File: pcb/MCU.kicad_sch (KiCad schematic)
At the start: 14 parts, among them U1 WeMos_S2_mini

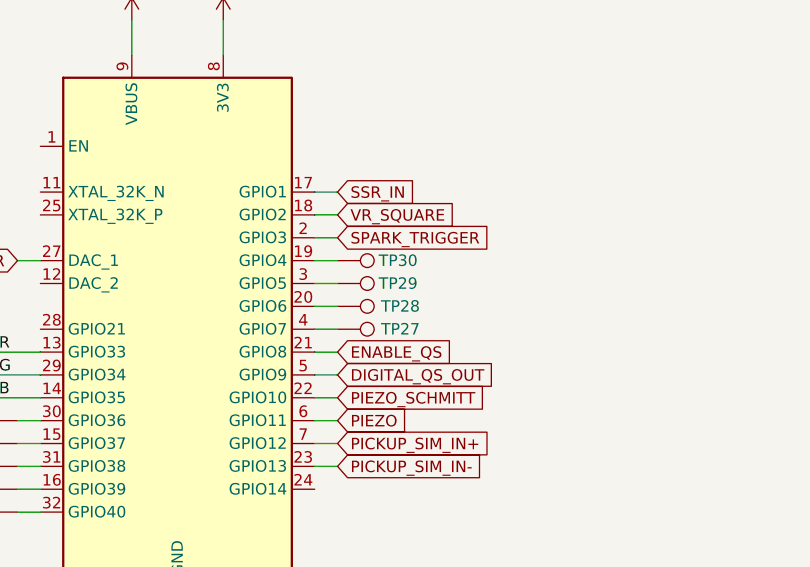
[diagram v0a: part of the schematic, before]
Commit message: added connector and simulation link
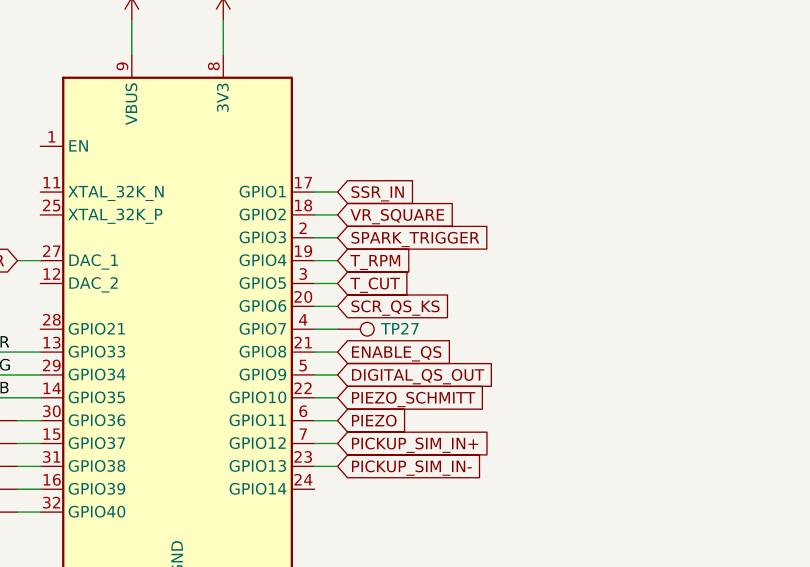
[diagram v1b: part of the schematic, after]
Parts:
- removed TP28, TP29, TP30: TestPoint, Connector_PinHeader_1.00mm:PinHeader_1x01_P1.00mm_Vertical, symbol Connector:TestPoint
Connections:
- net SCR_QS_KS: now reaches U1.20 (GPIO6)
- net T_RPM: now reaches U1.19 (GPIO4)
- net T_CUT: now reaches U1.3 (GPIO5)
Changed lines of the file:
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@@
+		)
+	)
+	(global_label "SCR_QS_KS"
+		(shape input)
+		(at 86.36 64.77 0)
+		(fields_autoplaced yes)
+		(effects
+			(font
+				(size 1.27 1.27)
+			)
+			(justify left)
+		)
+		(property "Intersheetrefs" "${INTERSHEET_REFS}"
+			(at 100.0494 64.77 0)
+			(effects
+				(font
+					(size 1.27 1.27)
+				)
+				(justify left)
+				(hide yes)
+			)
 		)
 	)
@@
 		)
 	)
+	(global_label "T_RPM"
+		(shape input)
+		(at 86.36 59.69 0)
+		(fields_autoplaced yes)
+		(effects
+			(font
+				(size 1.27 1.27)
+			)
+			(justify left)
+		)
+		(property "Intersheetrefs" "${INTERSHEET_REFS}"
+			(at 95.2718 59.69 0)
+			(effects
+				(font
+					(size 1.27 1.27)
+				)
+				(justify left)
+				(hide yes)
+			)
+		)
+	)
+	(global_label "T_CUT"
+		(shape input)
+		(at 86.36 62.23 0)
+		(fields_autoplaced yes)
+		(effects
+			(font
+				(size 1.27 1.27)
+			)
+			(justify left)
+		)
+		(property "Intersheetrefs" "${INTERSHEET_REFS}"
+			(at 94.8485 62.23 0)
+			(effects
+				(font
+					(size 1.27 1.27)
+				)
+				(justify left)
+				(hide yes)
+			)
+		)
+	)
 	(global_label "PWM_VR"
 		(shape input)
@@
 	)
 	(symbol
-		(lib_id "Connector:TestPoint")
-		(at 86.36 64.77 270)
-		(unit 1)
-		(exclude_from_sim no)
-		(in_bom yes)
-		(on_board yes)
-		(dnp no)
-		(property "Reference" "TP28"
-			(at 91.186 64.77 90)
-			(effects
-				(font
-					(size 1.27 1.27)
-				)
-				(justify left)
-			)
-		)
-		(property "Value" "TestPoint"
-			(at 88.3921 67.31 0)
-			(effects
-				(font
-					(size 1.27 1.27)
-				)
-				(justify left)
-				(hide yes)
-			)
-		)
-		(property "Footprint" "Connector_PinHeader_1.00mm:PinHeader_1x01_P1.00mm_Vertical"
-			(at 86.36 69.85 0)
-			(effects
-				(font
-					(size 1.27 1.27)
-				)
-				(hide yes)
-			)
-		)
-		(property "Datasheet" "~"
-			(at 86.36 69.85 0)
-			(effects
-				(font
-					(size 1.27 1.27)
-				)
-				(hide yes)
-			)
-		)
-		(property "Description" "test point"
-			(at 86.36 64.77 0)
-			(effects
-				(font
-					(size 1.27 1.27)
-				)
-				(hide yes)
-			)
-		)
-		(pin "1"
-		)
-		(instances
-			(project "ecu-dev-board"
-				(path "/38d4df77-b5a0-4642-8410-8b13c21c2c3b/5baacb37-d82a-49c1-a6be-f8a839583d33"
-					(reference "TP28")
-					(unit 1)
-				)
-			)
-		)
-	)
-	(symbol
 		(lib_id "power:GND")
 		(at 265.43 52.07 0)
@@
 	)
 	(symbol
-		(lib_id "Connector:TestPoint")
-		(at 86.36 59.69 270)
-		(unit 1)
-		(exclude_from_sim no)
-		(in_bom yes)
-		(on_board yes)
-		(dnp no)
-		(property "Reference" "TP30"
-			(at 90.932 59.69 90)
-			(effects
-				(font
-					(size 1.27 1.27)
-				)
-				(justify left)
-			)
-		)
-		(property "Value" "TestPoint"
-			(at 88.3921 62.23 0)
-			(effects
-				(font
-					(size 1.27 1.27)
-				)
-				(justify left)
-				(hide yes)
-			)
-		)
-		(property "Footprint" "Connector_PinHeader_1.00mm:PinHeader_1x01_P1.00mm_Vertical"
-			(at 86.36 64.77 0)
-			(effects
-				(font
-					(size 1.27 1.27)
-				)
-				(hide yes)
-			)
-		)
-		(property "Datasheet" "~"
-			(at 86.36 64.77 0)
-			(effects
-				(font
-					(size 1.27 1.27)
-				)
-				(hide yes)
-			)
-		)
-		(property "Description" "test point"
-			(at 86.36 59.69 0)
-			(effects
-				(font
-					(size 1.27 1.27)
-				)
-				(hide yes)
-			)
-		)
-		(pin "1"
-		)
-		(instances
-			(project "ecu-dev-board"
-				(path "/38d4df77-b5a0-4642-8410-8b13c21c2c3b/5baacb37-d82a-49c1-a6be-f8a839583d33"
-					(reference "TP30")
-					(unit 1)
-				)
-			)
-		)
-	)
-	(symbol
 		(lib_id "power:GND")
 		(at 68.58 101.6 0)
@@
 					(unit 1)
 				)
-			)
-		)
-	)
-	(symbol
-		(lib_id "Connector:TestPoint")
-		(at 86.36 62.23 270)
-		(unit 1)
-		(exclude_from_sim no)
-		(in_bom yes)
-		(on_board yes)
-		(dnp no)
-		(property "Reference" "TP29"
-			(at 90.932 62.23 90)
-			(effects
-				(font
-					(size 1.27 1.27)
-				)
-				(justify left)
-			)
-		)
-		(property "Value" "TestPoint"
-			(at 88.3921 64.77 0)
-			(effects
-				(font
-					(size 1.27 1.27)
-				)
-				(justify left)
-				(hide yes)
-			)
-		)
-		(property "Footprint" "Connector_PinHeader_1.00mm:PinHeader_1x01_P1.00mm_Vertical"
-			(at 86.36 67.31 0)
-			(effects
-				(font
-					(size 1.27 1.27)
-				)
-				(hide yes)
-			)
-		)
-		(property "Datasheet" "~"
-			(at 86.36 67.31 0)
-			(effects
-				(font
-					(size 1.27 1.27)
-				)
-				(hide yes)
-			)
-		)
-		(property "Description" "test point"
-			(at 86.36 62.23 0)
-			(effects
-				(font
-					(size 1.27 1.27)
-				)
-				(hide yes)
-			)
-		)
-		(pin "1"
-		)
-		(instances
-			(project "ecu-dev-board"
-				(path "/38d4df77-b5a0-4642-8410-8b13c21c2c3b/5baacb37-d82a-49c1-a6be-f8a839583d33"
-					(reference "TP29")
-					(unit 1)
-				)
